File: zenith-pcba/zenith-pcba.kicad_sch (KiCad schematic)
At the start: 2 parts, among them U1 XC7A50T-CSG325, U2 K4B4G1646E-BCNB

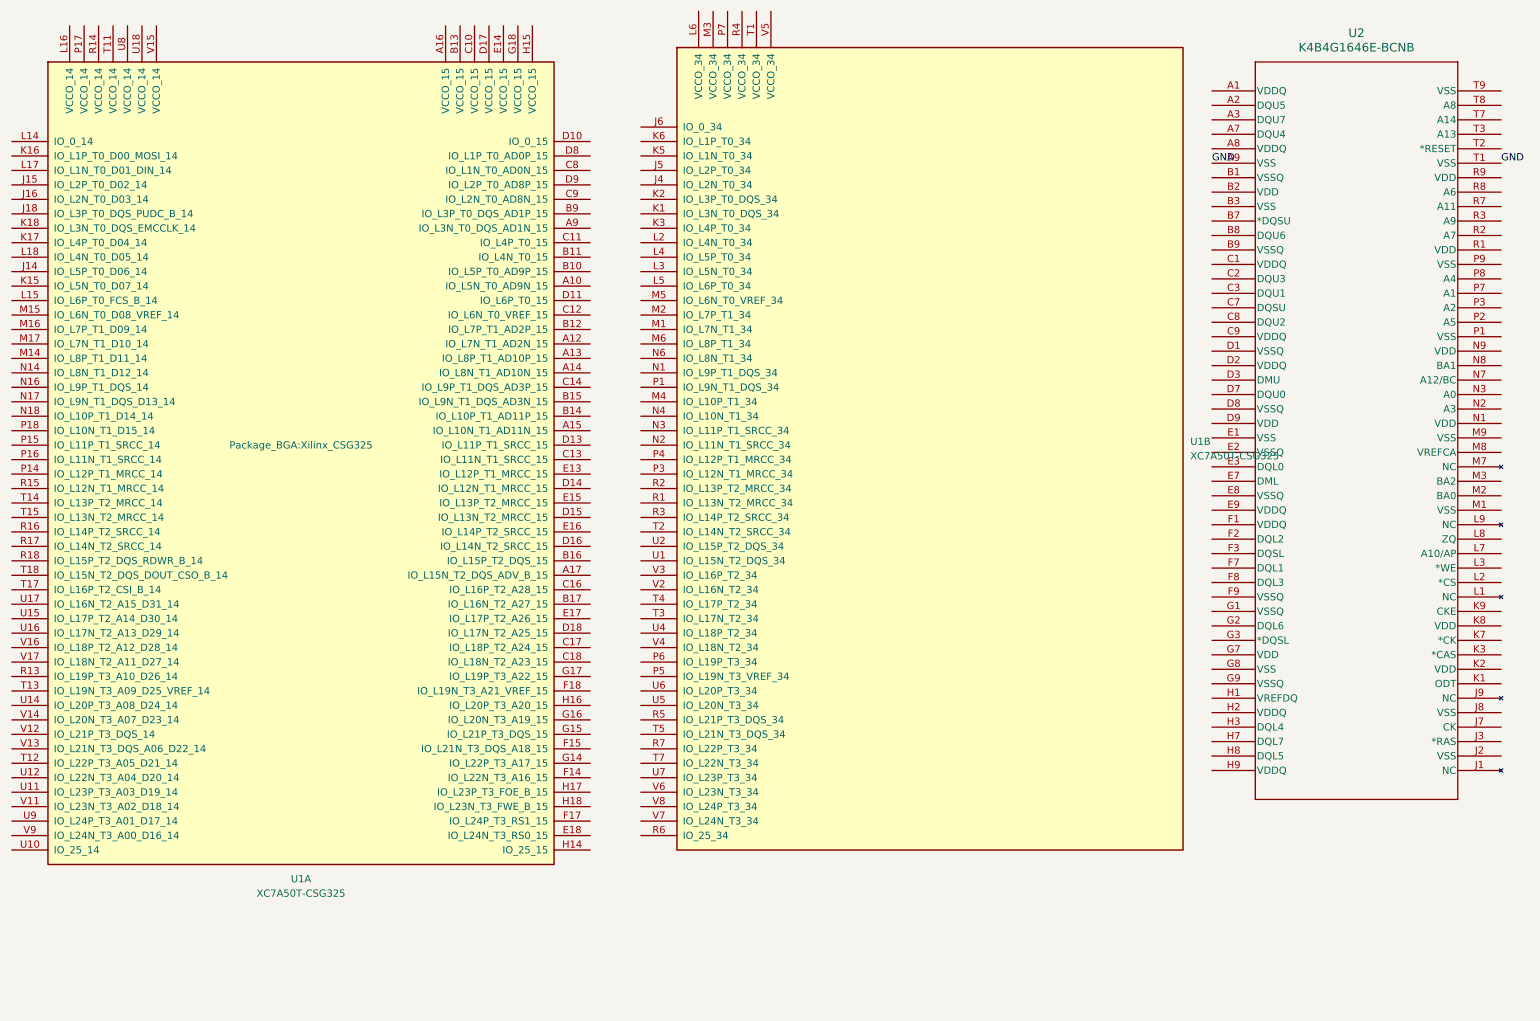
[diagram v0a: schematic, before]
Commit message: feat(pcba): initial programmer setup
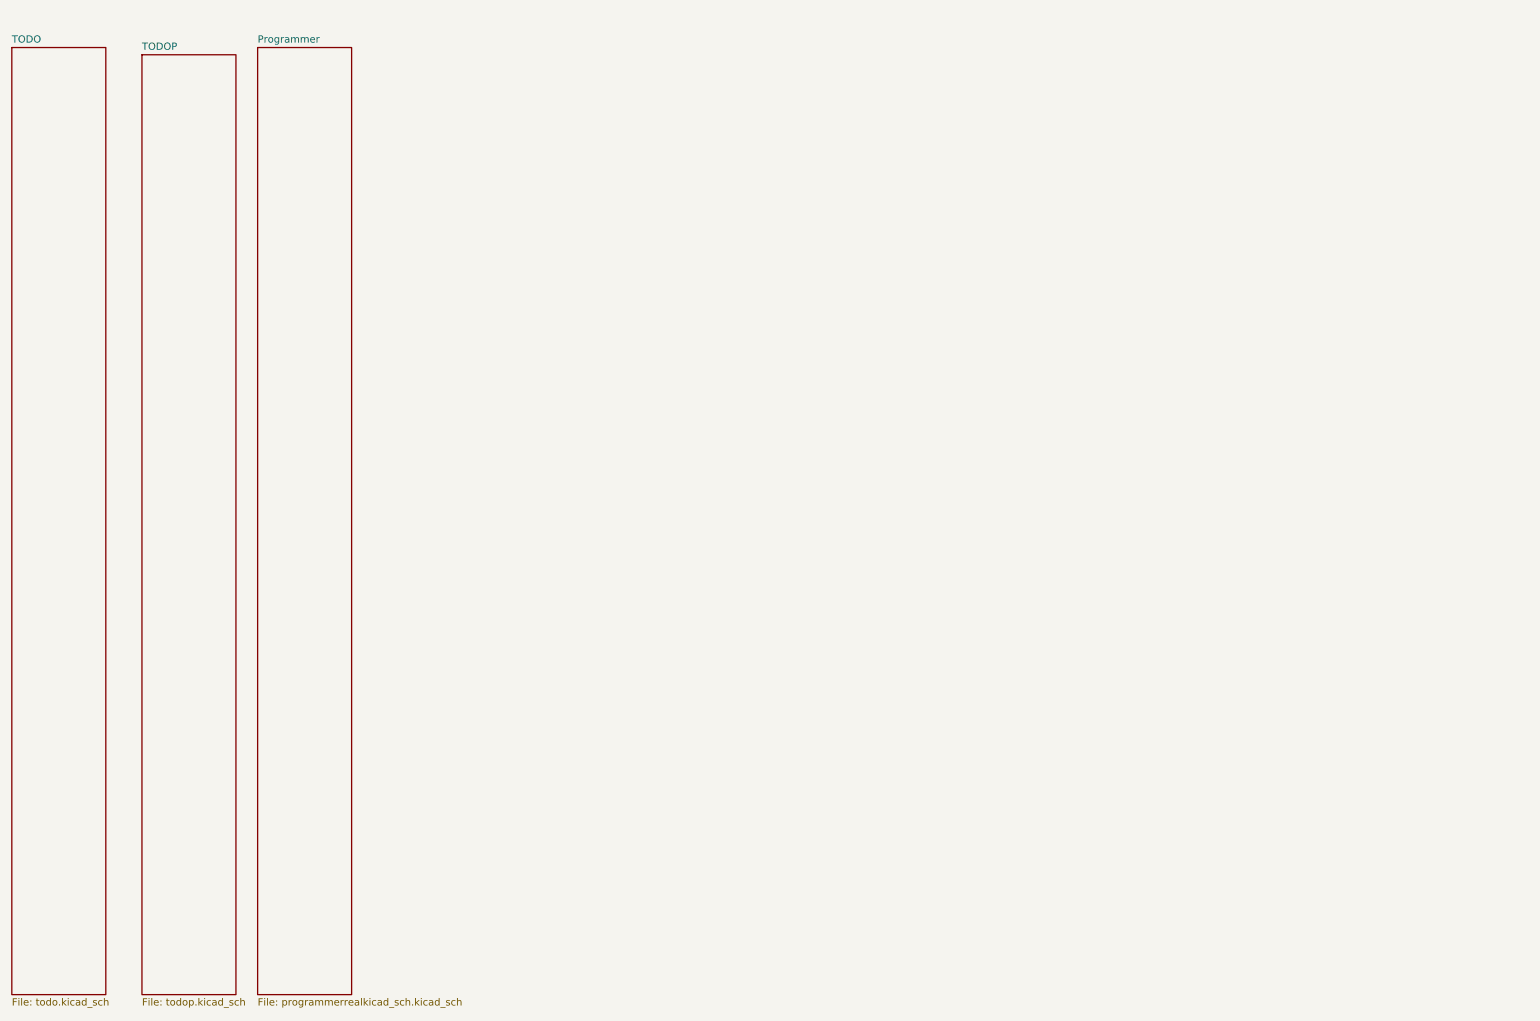
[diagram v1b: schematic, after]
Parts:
- removed U1: XC7A50T-CSG325, Package_BGA:Xilinx_CSG325, symbol FPGA_Xilinx_Artix7:XC7A50T-CSG325
- removed U2: K4B4G1646E-BCNB, BGA96_K4B4G1_SAM, symbol K4B4G1646E-BCNB:K4B4G1646E-BCNB
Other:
- added sheet Programmer (programmerrealkicad_sch.kicad_sch)
- added sheet TODO (todo.kicad_sch)
- added sheet TODOP (todop.kicad_sch)
